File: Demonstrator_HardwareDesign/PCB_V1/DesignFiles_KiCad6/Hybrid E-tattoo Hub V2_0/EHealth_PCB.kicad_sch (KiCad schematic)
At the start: 54 parts, among them J1 Conn_01x06, J2 Conn_01x06, J3 Conn_01x06, J3-MagneticInterconnect1 Conn_01x08, J4 Conn_01x06, J4-OffTheShelf-Digital1 Conn_02x06_Counter_Clockwise, J5-Power1 Conn_01x03, J5-Power2 Conn_01x03, T1 BSC320N20NS3_G, U1 TCA9548APWR, U2 DEBO DCDC DOWN 4

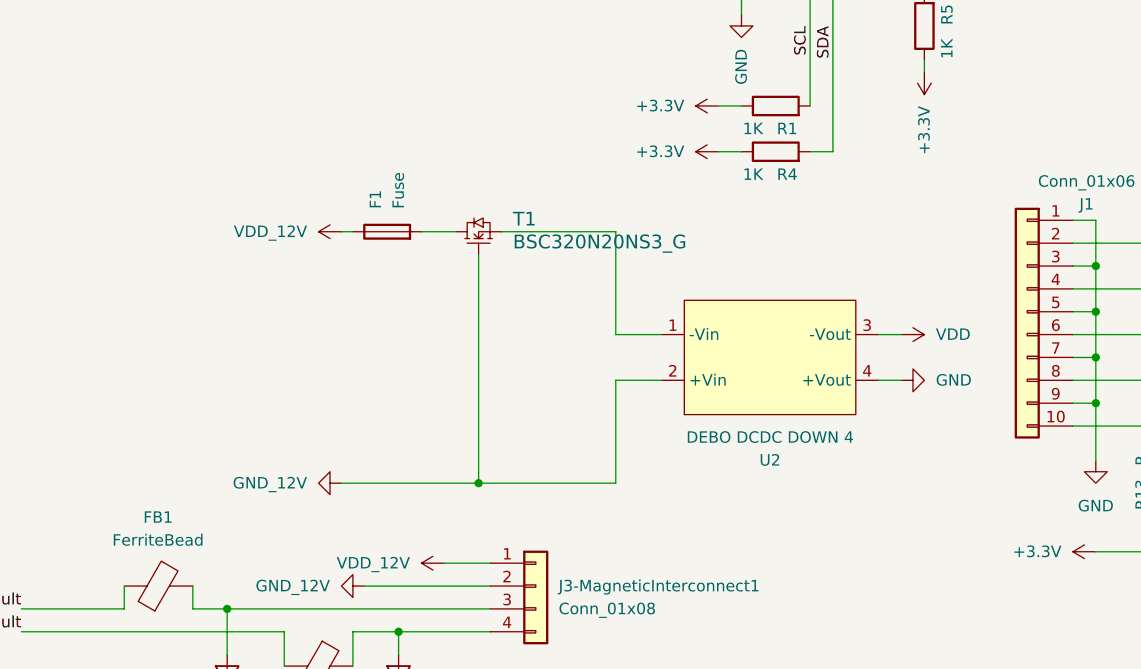
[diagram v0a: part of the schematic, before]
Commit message: up to date
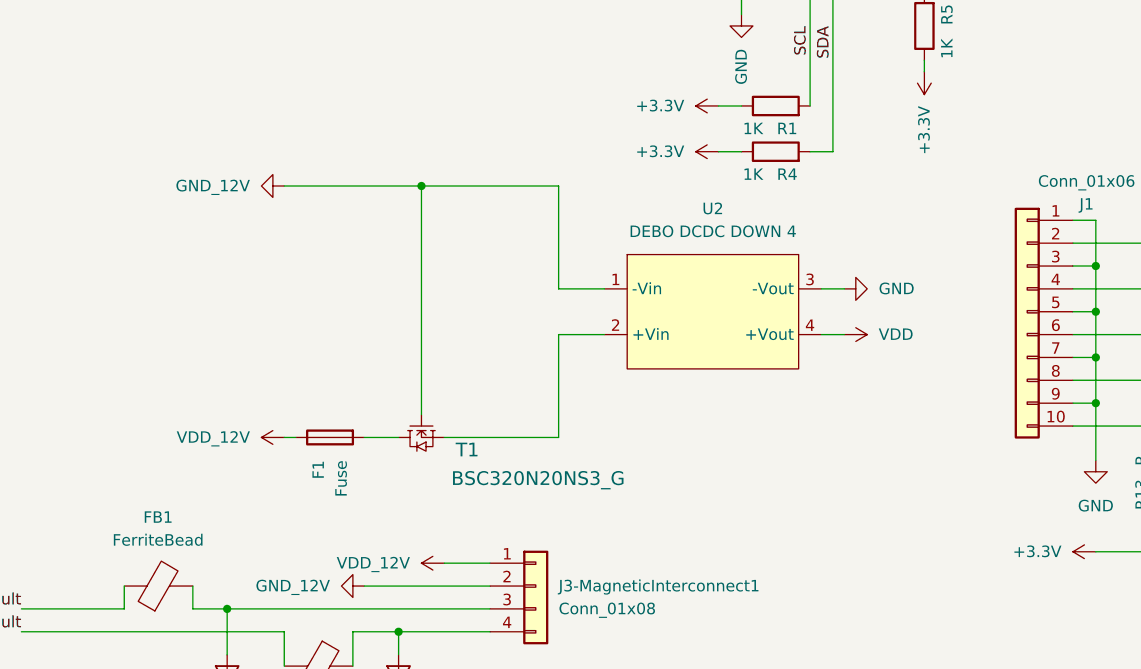
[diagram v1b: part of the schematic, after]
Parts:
- T1: footprint Library-TRANS:PG-TDSON-8 -> Package_SON:Infineon_PG-TDSON-8_6.15x5.15mm
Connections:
- net GND: now also U2.3 (-Vout); no longer U2.4 (+Vout)
- net GND_12V: now also U2.1 (-Vin); no longer U2.2 (+Vin)
- net VDD: now also U2.4 (+Vout); no longer U2.3 (-Vout)
- net at T1.1 (S): now also U2.2 (+Vin); no longer U2.1 (-Vin)
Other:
- moved on the sheet: U2
